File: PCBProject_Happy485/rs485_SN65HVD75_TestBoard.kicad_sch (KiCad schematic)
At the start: 12 parts, among them J1 UART_CONNECT, J2 RS485_CONNECT, J3 RS485_CONNECT, U1 SN65HVD75D

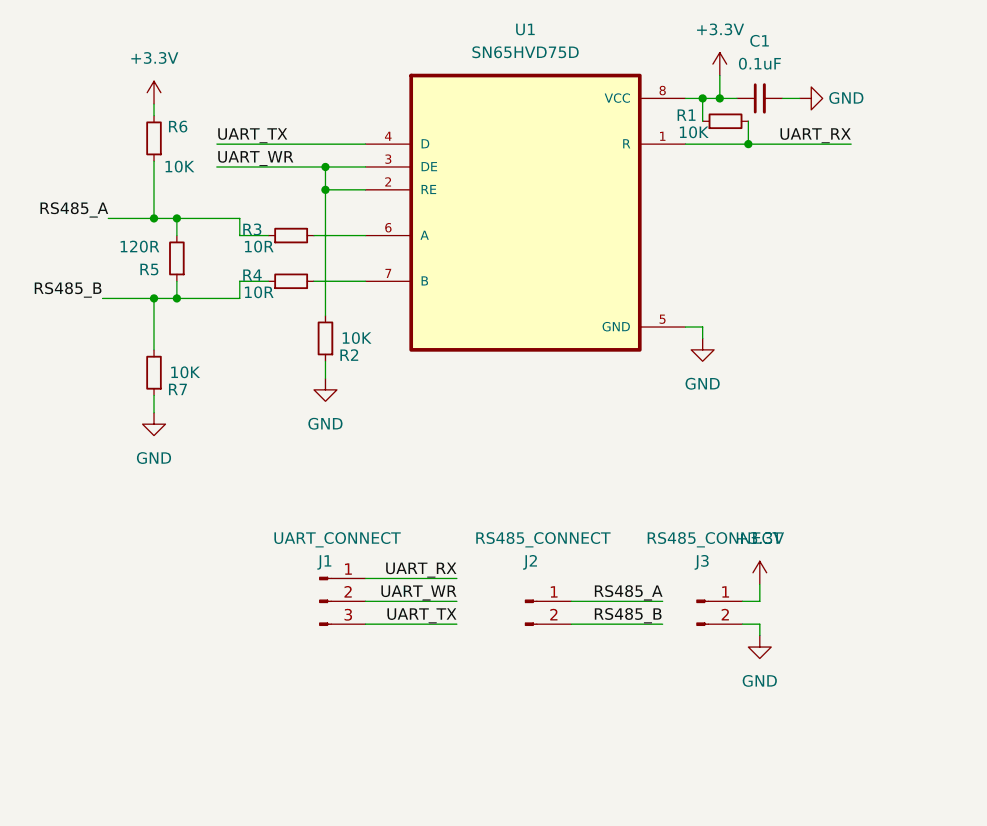
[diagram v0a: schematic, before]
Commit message: finish happy485
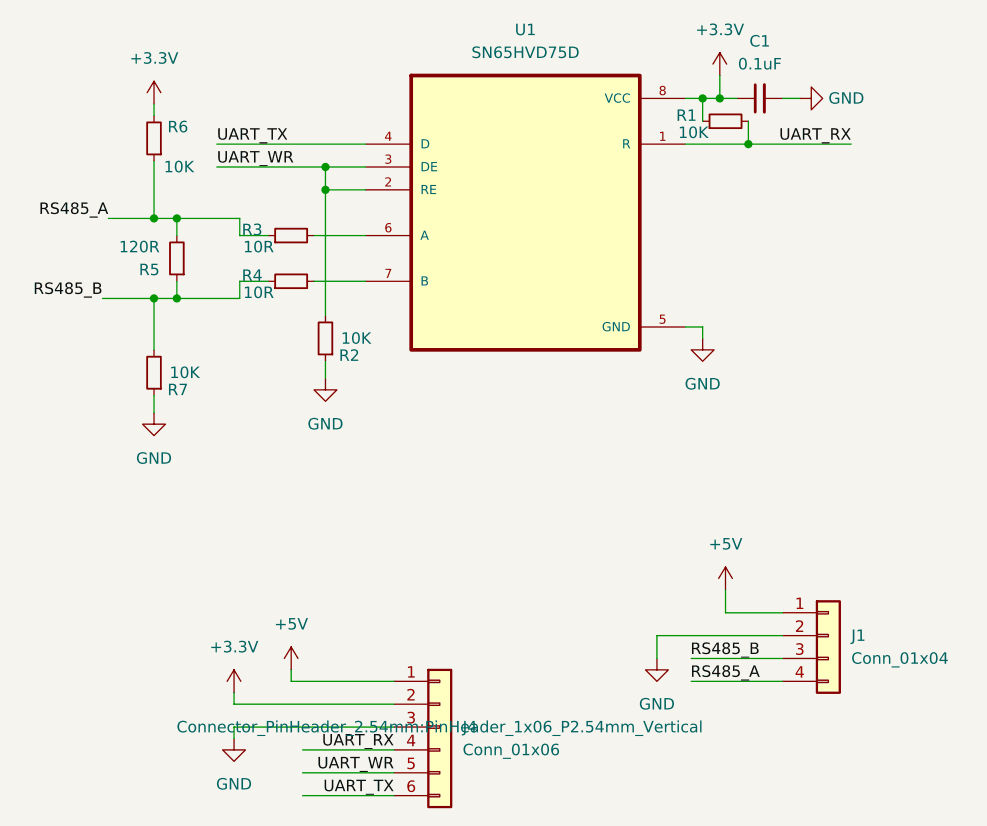
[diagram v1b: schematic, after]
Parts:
- removed J1: UART_CONNECT, Connector_PinSocket_2.54mm:PinSocket_1x03_P2.54mm_Vertical, symbol Connector:Conn_01x03_Pin
- removed J2, J3: RS485_CONNECT, Connector_PinSocket_2.54mm:PinSocket_1x02_P2.54mm_Vertical, symbol Connector:Conn_01x02_Pin
- added J1: Conn_01x04, Connector_PinHeader_2.54mm:PinHeader_1x04_P2.54mm_Vertical, symbol Connector_Generic:Conn_01x04
- added J4: Conn_01x06, Connector_PinHeader_2.54mm:PinHeader_1x06_P2.54mm_Vertical, symbol Connector_Generic:Conn_01x06
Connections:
- net +3.3V: now also J4.2 (Pin_2)
- net GND: now also J1.2 (Pin_2), J4.3 (Pin_3)
- net RS485_A: now also J1.4 (Pin_4)
- net RS485_B: now also J1.3 (Pin_3)
- net UART_RX: now also J4.4 (Pin_4)
- net UART_TX: now also J4.6 (Pin_6)
- net UART_WR: now also J4.5 (Pin_5)
- new net +5V: J1.1 (Pin_1), J4.1 (Pin_1)
